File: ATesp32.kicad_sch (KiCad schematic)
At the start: 22 parts, among them SW1 SW_Push, SW2 SW_Push, U1 ESP32-S3, U2 ATmega32A-P, Y1 40 MHz

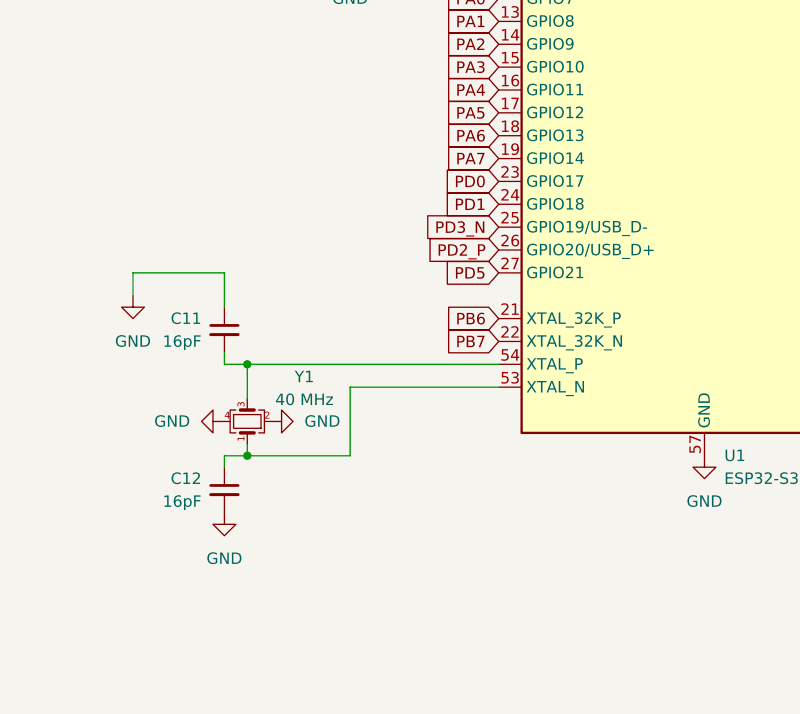
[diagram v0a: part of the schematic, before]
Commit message: Finished layout, need to fix silk
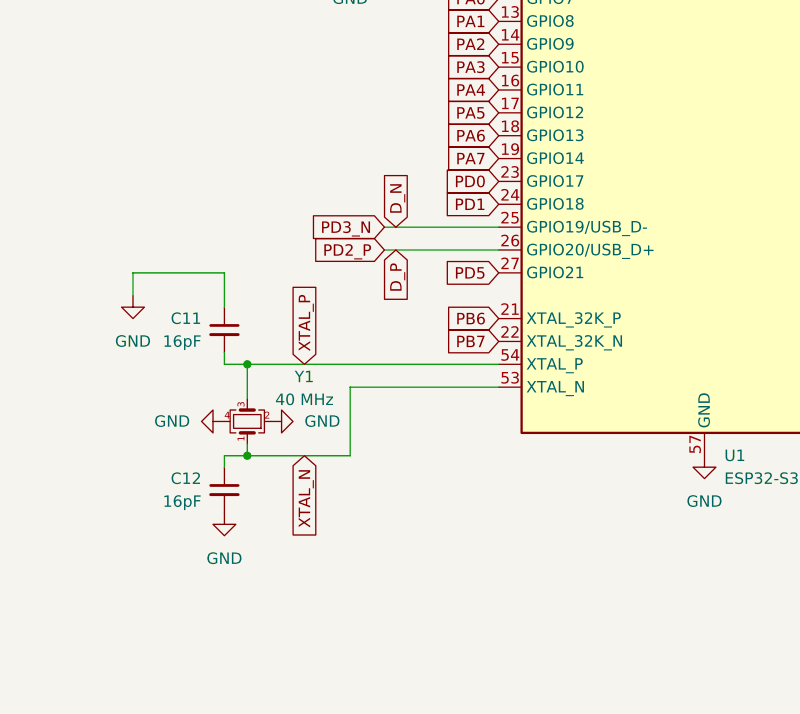
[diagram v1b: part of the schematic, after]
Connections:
- net XTAL_N: now reaches C12.1, U1.53 (XTAL_N), Y1.1
- net XTAL_P: now reaches C11.2, U1.54 (XTAL_P), Y1.3
- net PD2_P renamed D_P
- net PD3_N renamed D_N
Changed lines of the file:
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@@
+	(wire
+		(pts
+			(xy 63.5 115.57) (xy 76.2 115.57)
+		)
+		(stroke
+			(width 0)
+			(type default)
+		)
+	)
 	(wire
 		(pts
@@
 		(pts
 			(xy 255.27 34.29) (xy 259.08 34.29)
+		)
+		(stroke
+			(width 0)
+			(type default)
+		)
+	)
+	(wire
+		(pts
+			(xy 63.5 113.03) (xy 76.2 113.03)
 		)
 		(stroke
@@
 		)
 	)
+	(global_label "XTAL_N"
+		(shape input)
+		(at 54.61 138.43 270)
+		(fields_autoplaced yes)
+		(effects
+			(font
+				(size 1.27 1.27)
+			)
+			(justify right)
+		)
+		(property "Intersheetrefs" "${INTERSHEET_REFS}"
+			(at 54.61 148.0071 90)
+			(effects
+				(font
+					(size 1.27 1.27)
+				)
+				(justify right)
+				(hide yes)
+			)
+		)
+	)
+	(global_label "XTAL_P"
+		(shape input)
+		(at 54.61 128.27 90)
+		(fields_autoplaced yes)
+		(effects
+			(font
+				(size 1.27 1.27)
+			)
+			(justify left)
+		)
+		(property "Intersheetrefs" "${INTERSHEET_REFS}"
+			(at 54.61 118.7534 90)
+			(effects
+				(font
+					(size 1.27 1.27)
+				)
+				(justify left)
+				(hide yes)
+			)
+		)
+	)
 	(global_label "PC0"
 		(shape input)
@@
 	(global_label "PD2_P"
 		(shape input)
-		(at 76.2 115.57 180)
-		(fields_autoplaced yes)
-		(effects
-			(font
-				(size 1.27 1.27)
-			)
-			(justify right)
-		)
-		(property "Intersheetrefs" "${INTERSHEET_REFS}"
-			(at 69.4653 115.57 0)
+		(at 63.5 115.57 180)
+		(fields_autoplaced yes)
+		(effects
+			(font
+				(size 1.27 1.27)
+			)
+			(justify right)
+		)
+		(property "Intersheetrefs" "${INTERSHEET_REFS}"
+			(at 56.7653 115.57 0)
 			(effects
 				(font
@@
 		)
 	)
+	(global_label "D_N"
+		(shape input)
+		(at 64.77 113.03 90)
+		(fields_autoplaced yes)
+		(effects
+			(font
+				(size 1.27 1.27)
+			)
+			(justify left)
+		)
+		(property "Intersheetrefs" "${INTERSHEET_REFS}"
+			(at 64.77 106.4767 90)
+			(effects
+				(font
+					(size 1.27 1.27)
+				)
+				(justify left)
+				(hide yes)
+			)
+		)
+	)
 	(global_label "PA2"
 		(shape input)
@@
 		)
 	)
+	(global_label "D_P"
+		(shape input)
+		(at 64.77 115.57 270)
+		(fields_autoplaced yes)
+		(effects
+			(font
+				(size 1.27 1.27)
+			)
+			(justify right)
+		)
+		(property "Intersheetrefs" "${INTERSHEET_REFS}"
+			(at 64.77 122.0628 90)
+			(effects
+				(font
+					(size 1.27 1.27)
+				)
+				(justify right)
+				(hide yes)
+			)
+		)
+	)
 	(global_label "PC3"
 		(shape input)
@@
 	(global_label "PD3_N"
 		(shape input)
-		(at 76.2 113.03 180)
-		(fields_autoplaced yes)
-		(effects
-			(font
-				(size 1.27 1.27)
-			)
-			(justify right)
-		)
-		(property "Intersheetrefs" "${INTERSHEET_REFS}"
-			(at 69.4653 113.03 0)
-			(effects
-				(font
+		(at 63.5 113.03 180)
+		(fields_autoplaced yes)
+		(effects
+			(font
+				(size 1.27 1.27)
+			)
+			(justify right)
+		)
+		(property "Intersheetrefs" "${INTERSHEET_REFS}"
+			(at 56.7653 113.03 0)
+			(effects
+				(font
